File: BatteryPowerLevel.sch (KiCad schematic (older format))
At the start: 18 parts, among them J1 Conn_01x02_Male, SW1 SW_Push

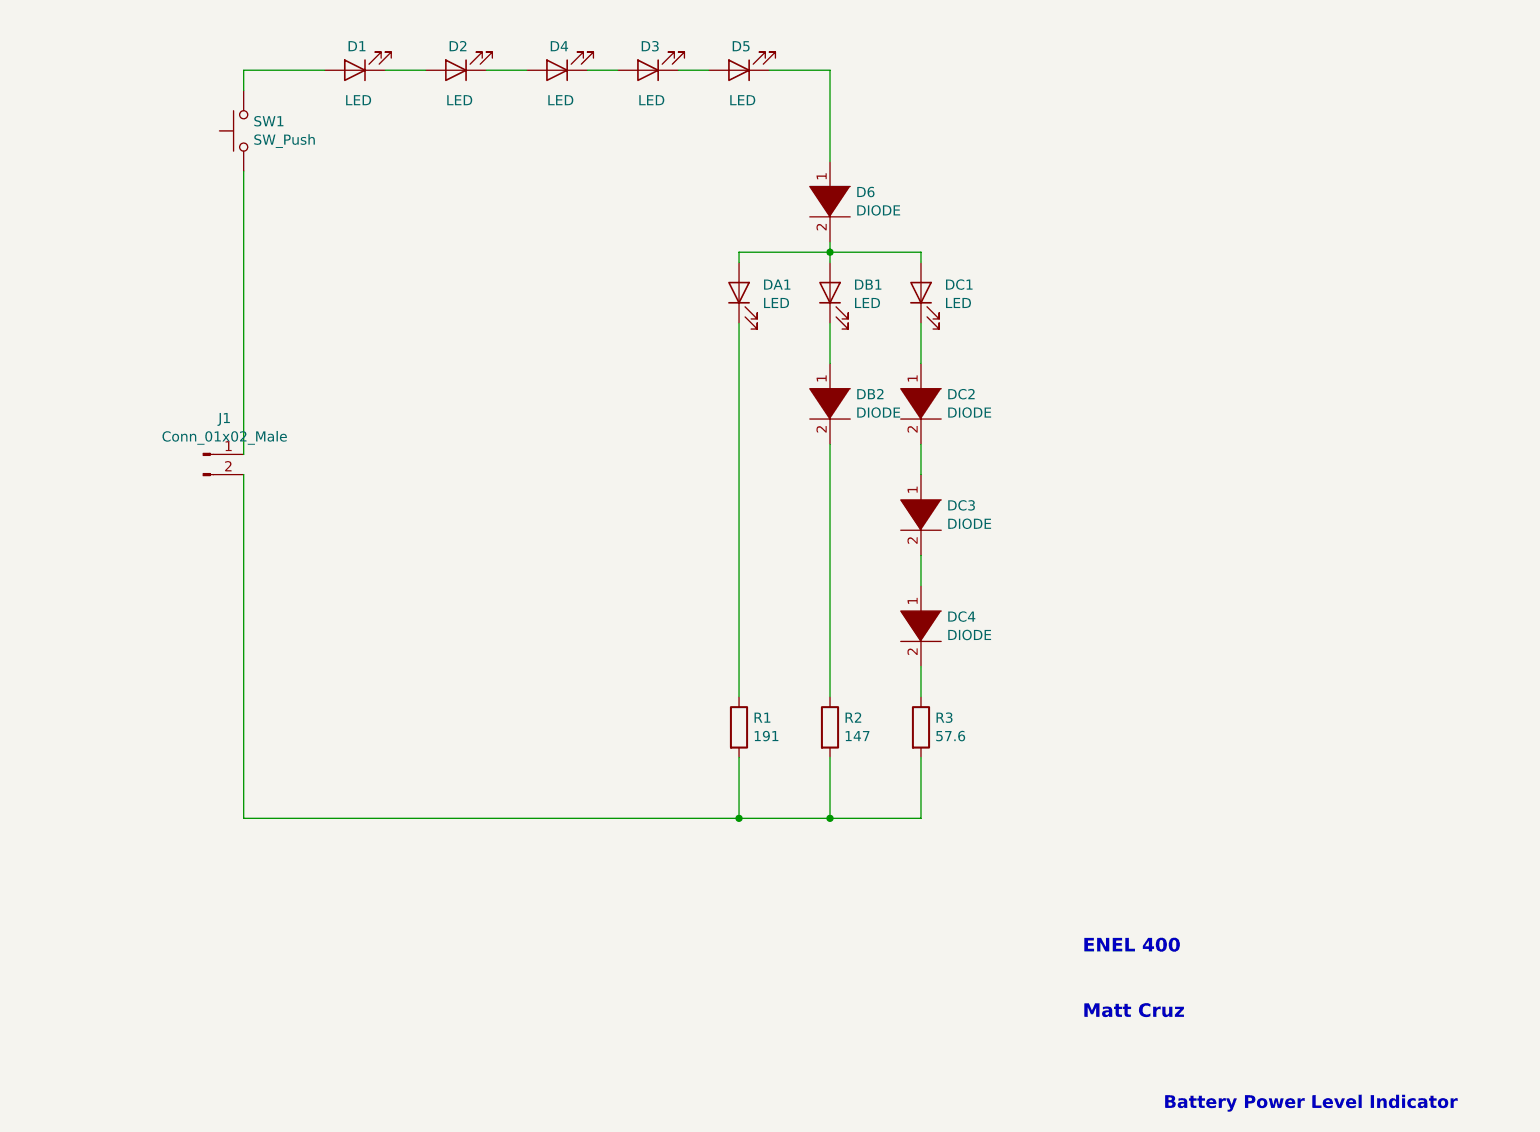
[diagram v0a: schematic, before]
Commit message: Revision
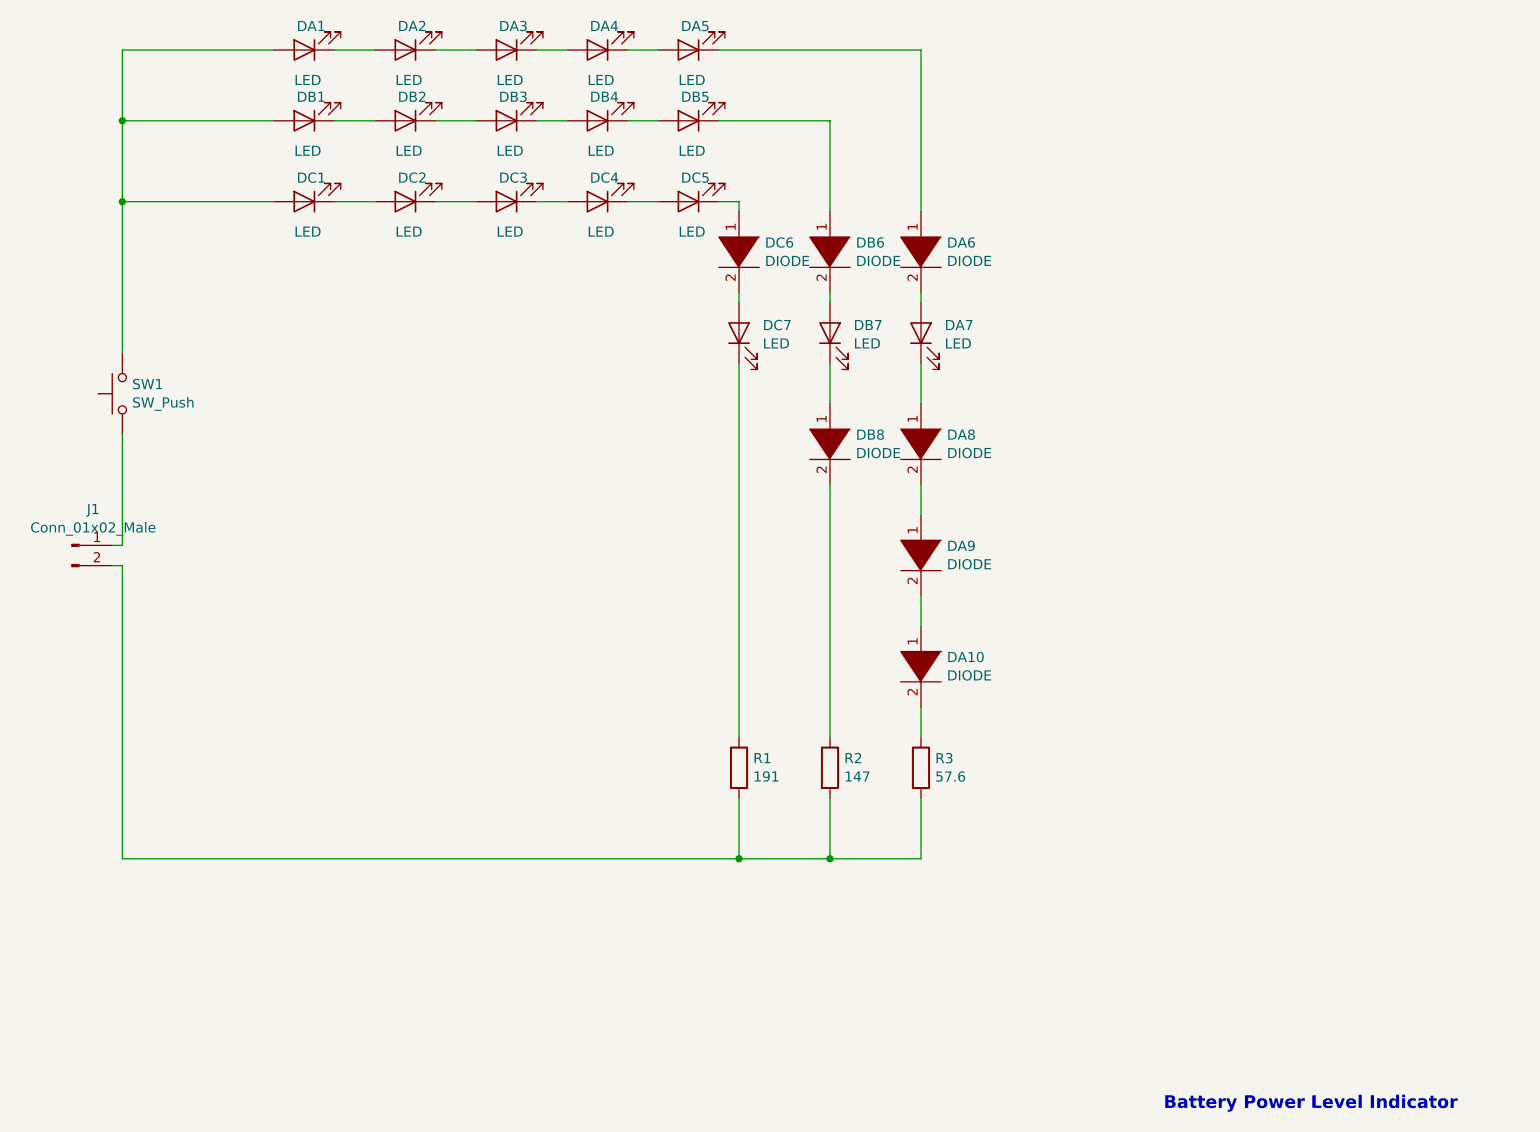
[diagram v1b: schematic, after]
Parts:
- added DA6, DC6: DIODE, Battery_Power_Level:CDSQR400B-HF (Diode 0.77V 10ohms), symbol pspice:DIODE
- added DB1, DB2, DB3, DB4, DB5, DC1, DC2, DC3, DC4, DC5: LED, Battery_Power_Level:LTST-C191KGKT (LED 2V), symbol Device:LED
- DA10: renamed from DC4; footprint Battery_Power_Level:MMBD914L (DIODE 0.77V) -> Battery_Power_Level:CDSQR400B-HF (Diode 0.77V 10ohms)
- DA8: renamed from DC2; footprint Battery_Power_Level:MMBD914L (DIODE 0.77V) -> Battery_Power_Level:CDSQR400B-HF (Diode 0.77V 10ohms)
- DA9: renamed from DC3; footprint Battery_Power_Level:MMBD914L (DIODE 0.77V) -> Battery_Power_Level:CDSQR400B-HF (Diode 0.77V 10ohms)
- DB6: renamed from D6; footprint Battery_Power_Level:MMBD914L (DIODE 0.77V) -> Battery_Power_Level:CDSQR400B-HF (Diode 0.77V 10ohms)
- DB8: renamed from DB2; footprint Battery_Power_Level:MMBD914L (DIODE 0.77V) -> Battery_Power_Level:CDSQR400B-HF (Diode 0.77V 10ohms)
- renumbered D1 to DA1, D2 to DA2, D4 to DA3, D3 to DA4, D5 to DA5, DC1 to DA7, DB1 to DB7, DA1 to DC7
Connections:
- net at DA1.2 (A), SW1.2: now also DB1.2 (A), DC1.2 (A)
- net at DA5.1 (K): now also DA6.1 (K); no longer DB6.1 (K)
- net at DB6.2 (A), DB7.2 (A): no longer DA7.2 (A), DC7.2 (A)
- new net: DC6.2 (A), DC7.2 (A)
- new net: DA6.2 (A), DA7.2 (A)
- new net: DB5.1 (K), DB6.1 (K)
- new net: DB1.1 (K), DB2.2 (A)
- new net: DB2.1 (K), DB3.2 (A)
- new net: DB4.1 (K), DB5.2 (A)
- new net: DB3.1 (K), DB4.2 (A)
- new net: DC1.1 (K), DC2.2 (A)
- new net: DC2.1 (K), DC3.2 (A)
- new net: DC4.1 (K), DC5.2 (A)
- new net: DC3.1 (K), DC4.2 (A)
- new net: DC5.1 (K), DC6.1 (K)
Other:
- note removed: "ENEL 400 \n\n\nMatt Cruz"
- moved on the sheet: DA1, DA10, DA2, DA3, DA4, DA5, DA7, DA8, DA9, DB6, DB7, DB8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

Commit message: Reverted
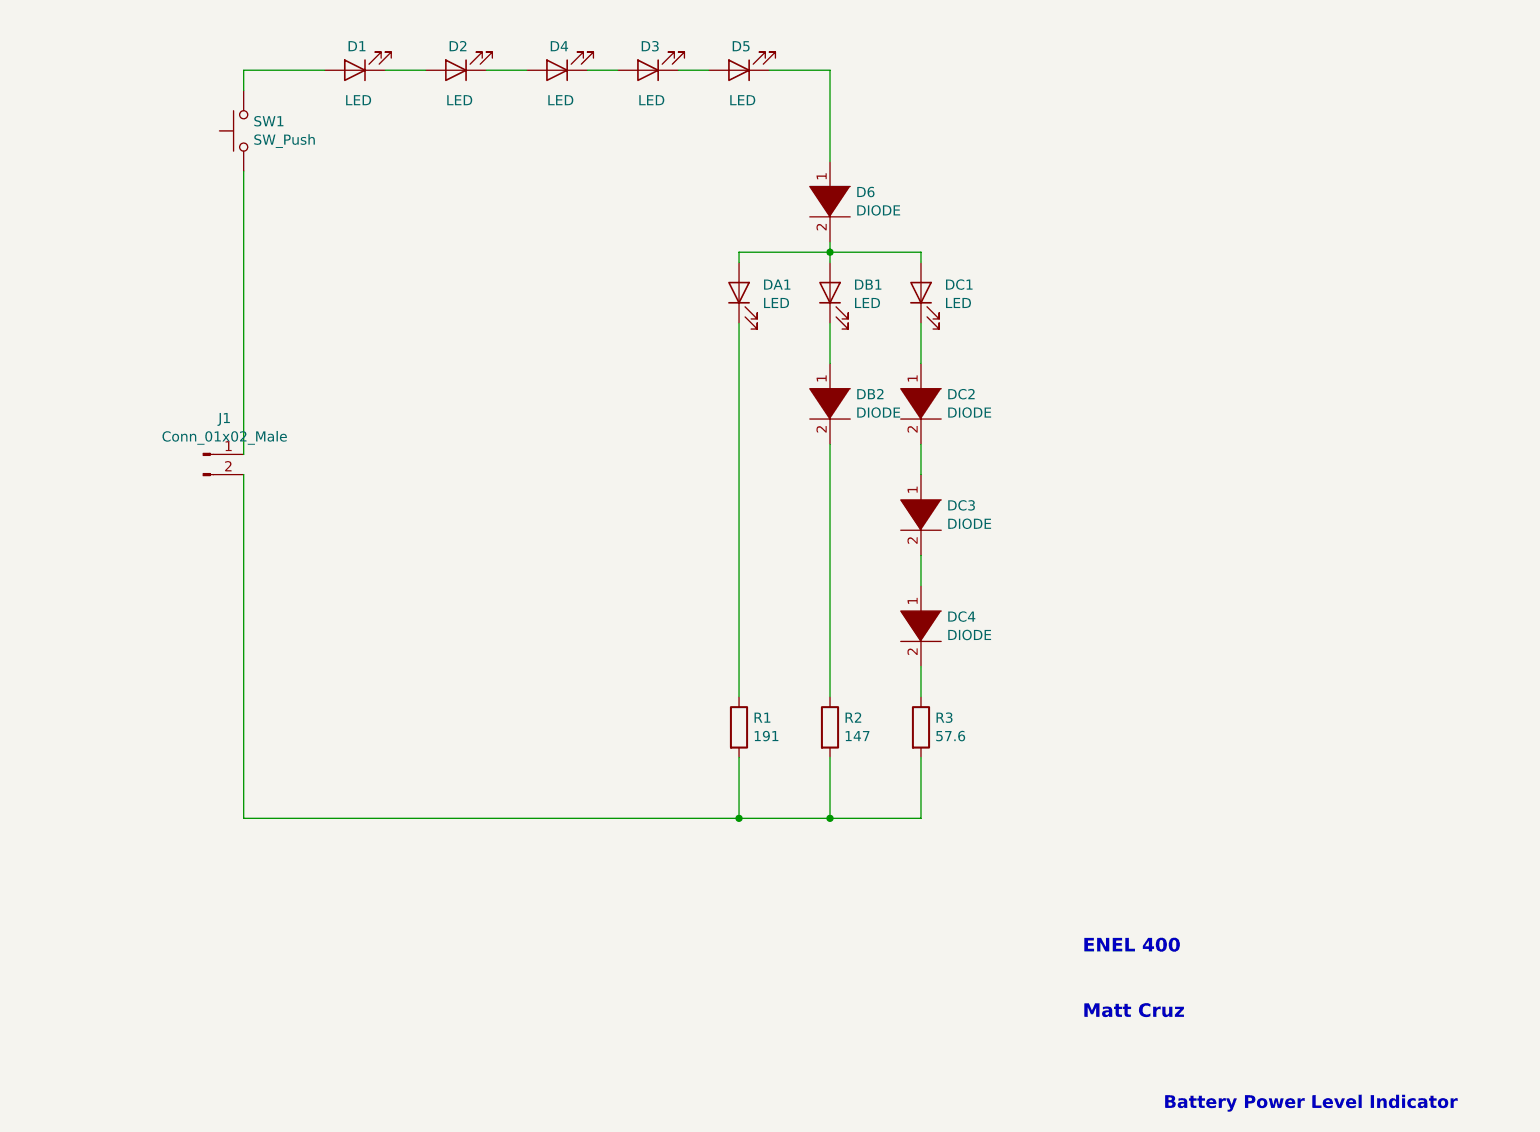
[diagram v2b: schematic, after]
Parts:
- removed DA6, DC6: DIODE, Battery_Power_Level:CDSQR400B-HF (Diode 0.77V 10ohms), symbol pspice:DIODE
- removed DB1, DB2, DB3, DB4, DB5, DC1, DC2, DC3, DC4, DC5: LED, Battery_Power_Level:LTST-C191KGKT (LED 2V), symbol Device:LED
- D6: renamed from DB6; footprint Battery_Power_Level:CDSQR400B-HF (Diode 0.77V 10ohms) -> Battery_Power_Level:MMBD914L (DIODE 0.77V)
- DB2: renamed from DB8; footprint Battery_Power_Level:CDSQR400B-HF (Diode 0.77V 10ohms) -> Battery_Power_Level:MMBD914L (DIODE 0.77V)
- DC2: renamed from DA8; footprint Battery_Power_Level:CDSQR400B-HF (Diode 0.77V 10ohms) -> Battery_Power_Level:MMBD914L (DIODE 0.77V)
- DC3: renamed from DA9; footprint Battery_Power_Level:CDSQR400B-HF (Diode 0.77V 10ohms) -> Battery_Power_Level:MMBD914L (DIODE 0.77V)
- DC4: renamed from DA10; footprint Battery_Power_Level:CDSQR400B-HF (Diode 0.77V 10ohms) -> Battery_Power_Level:MMBD914L (DIODE 0.77V)
- renumbered DA1 to D1, DA2 to D2, DA4 to D3, DA3 to D4, DA5 to D5, DC7 to DA1, DB7 to DB1, DA7 to DC1
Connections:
- net at D5.1 (K): now also D6.1 (K)
- net at D6.2 (A), DB1.2 (A): now also DA1.2 (A), DC1.2 (A)
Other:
- note added: "ENEL 400 \n\n\nMatt Cruz"
- moved on the sheet: D1, D2, D3, D4, D5, D6, DA1, DB1, DB2, DC1, DC2, DC3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
